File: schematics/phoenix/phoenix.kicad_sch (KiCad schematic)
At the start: 3 parts, among them U1 MAX31856

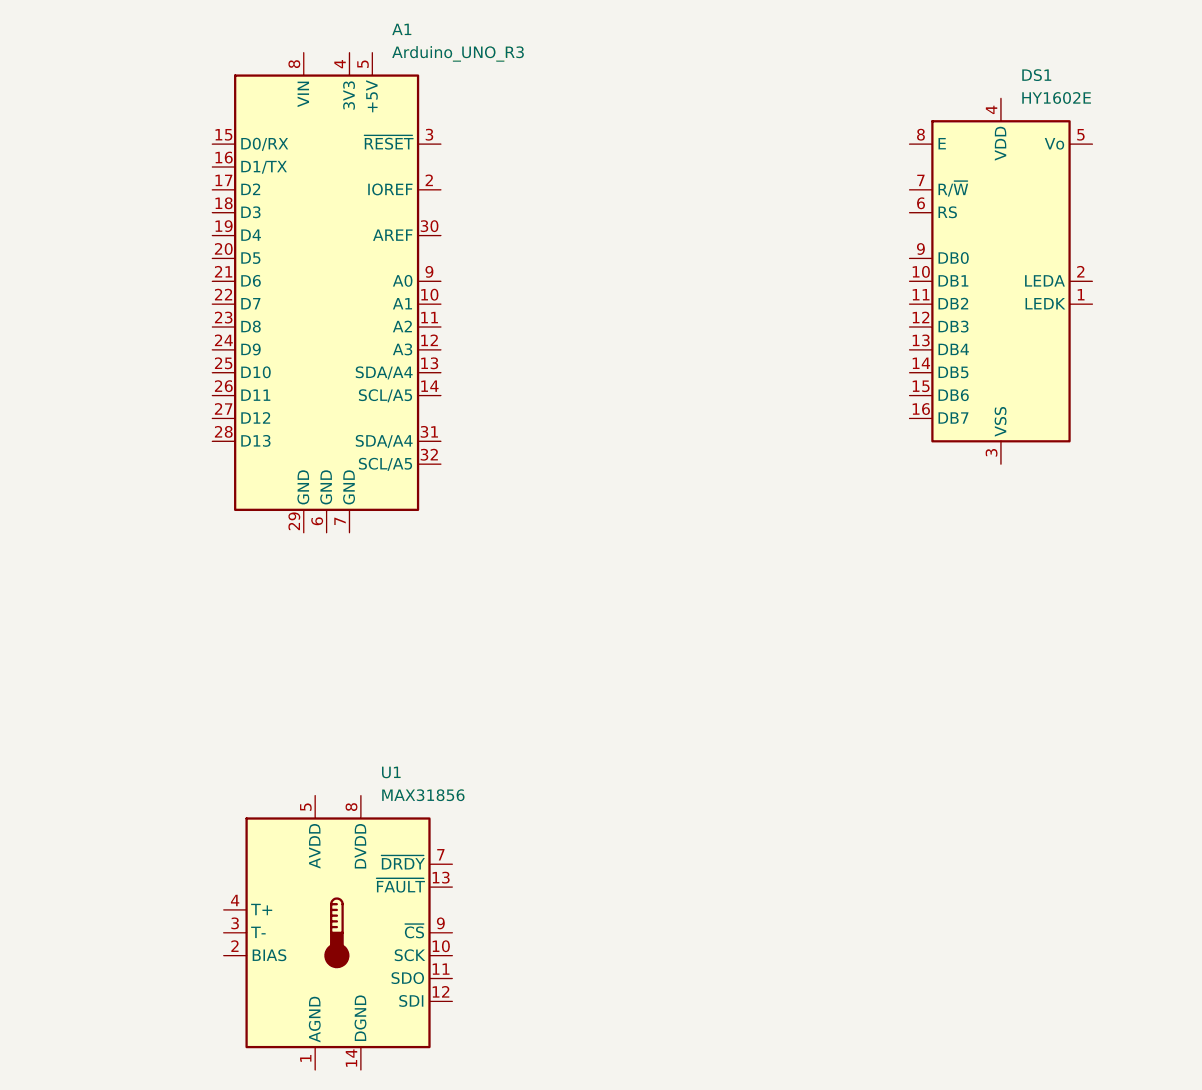
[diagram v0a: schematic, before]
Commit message: schematic updates
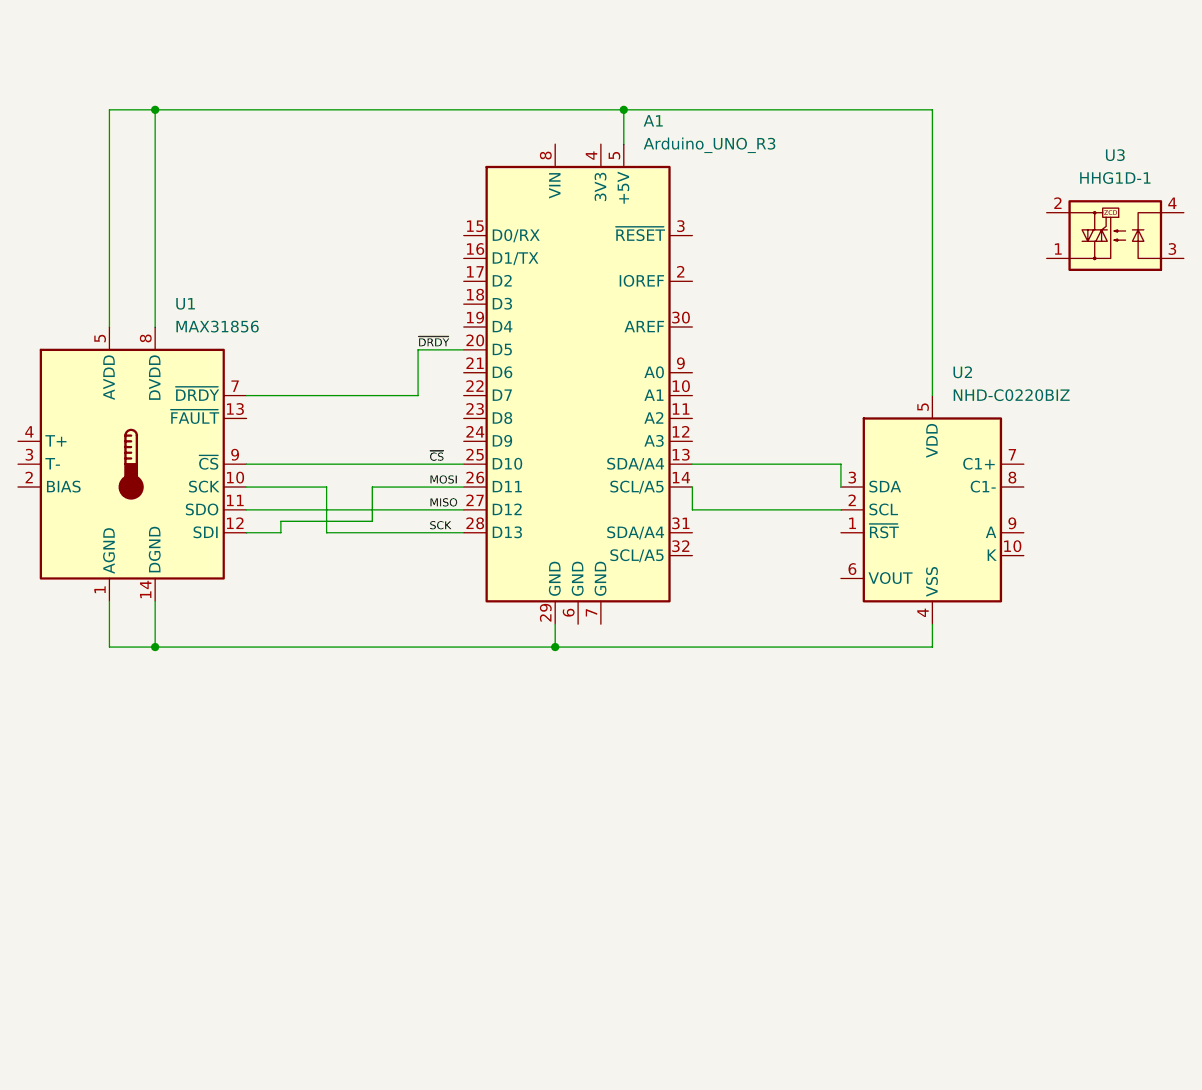
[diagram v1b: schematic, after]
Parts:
- removed DS1: HY1602E, Display:HY1602E, symbol Display_Character:HY1602E
- added U2: NHD-C0220BIZ, Package_DIP:DIP-20_W7.62mm_Socket, symbol Display_Character:NHD-C0220BIZ
- added U3: HHG1D-1, Relay_THT:Relay_NCR_HHG1D-1, symbol Relay_SolidState:HHG1D-1
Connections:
- net at U1.1 (AGND): now also A1.29 (GND), U1.14 (DGND), U2.4 (VSS)
- net SCK: now reaches U1.10 (SCK)
- net SCK: now also A1.28 (D13)
- net MISO: now reaches U1.11 (SDO)
- net MISO: now also A1.27 (D12)
- net MOSI: now reaches U1.12 (SDI)
- net MOSI: now also A1.26 (D11)
- net at U1.5 (AVDD): now also A1.5 (+5V), U1.8 (DVDD), U2.5 (VDD)
- net ~{DRDY}: now reaches U1.7 (~{DRDY})
- net ~{DRDY}: now also A1.20 (D5)
- net ~{CS}: now reaches U1.9 (~{CS})
- net ~{CS}: now also A1.25 (D10)
- net at A1.13 (SDA/A4): now also U2.3 (SDA)
- net at A1.14 (SCL/A5): now also U2.2 (SCL)
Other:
- moved on the sheet: A1, U1
